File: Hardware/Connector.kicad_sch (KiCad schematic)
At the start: 13 parts, among them J1 XIAO ESP32S3 Sense, J2 Conn_02x16_Counter_Clockwise, J3 FTSH-107-01-L-D-K

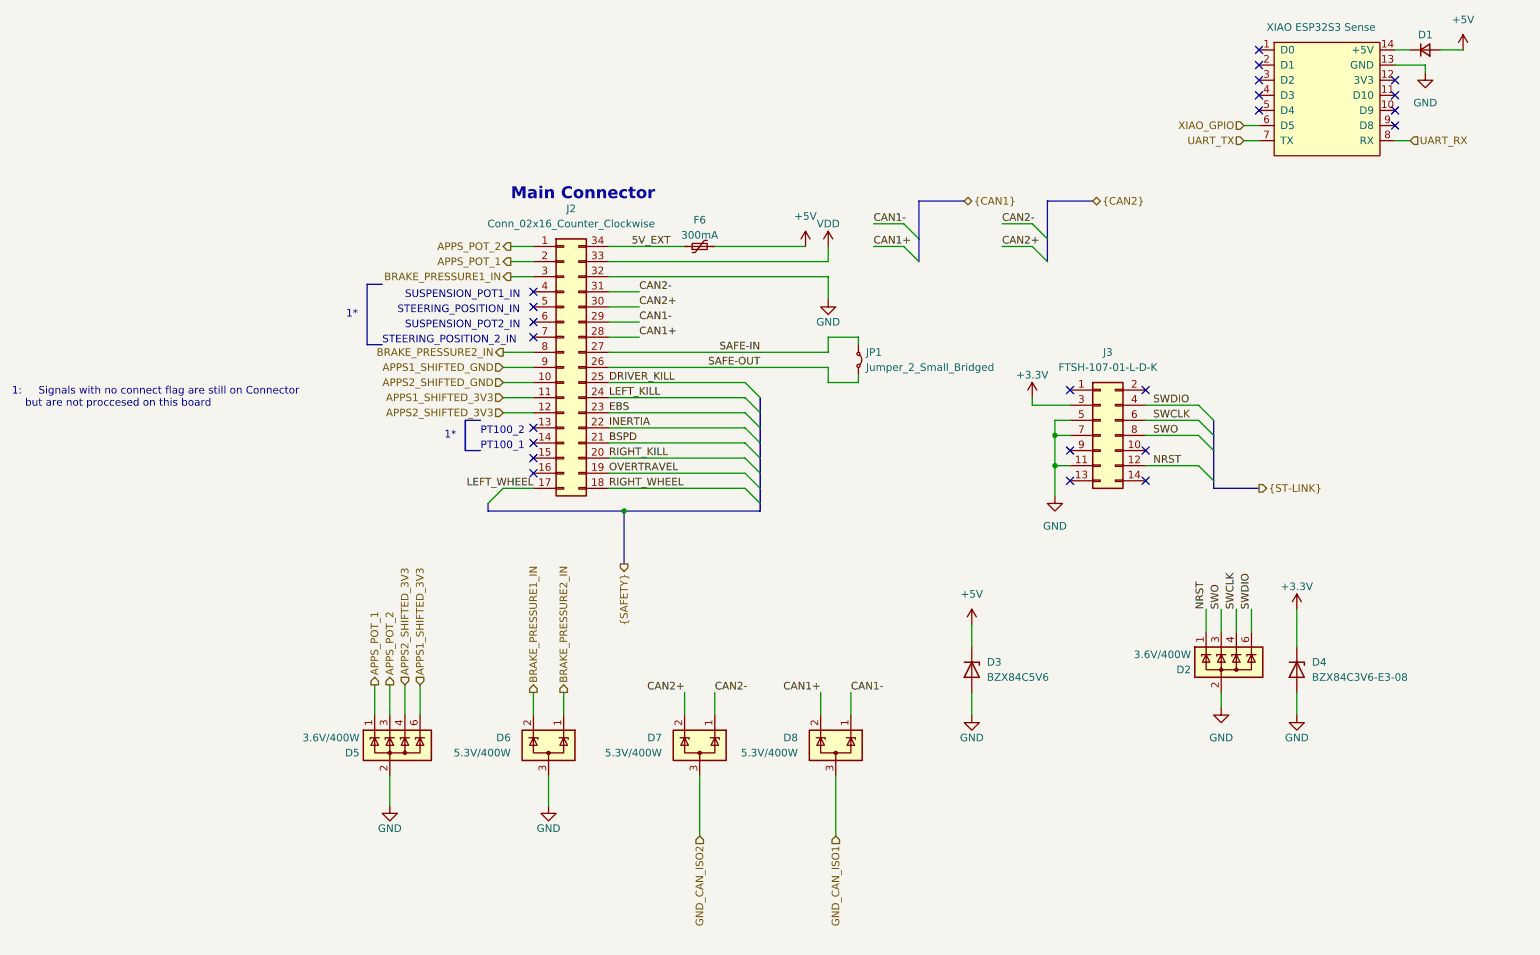
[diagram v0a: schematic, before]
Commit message: Initial routing (Piotruś proszę nie bij że brzydko)
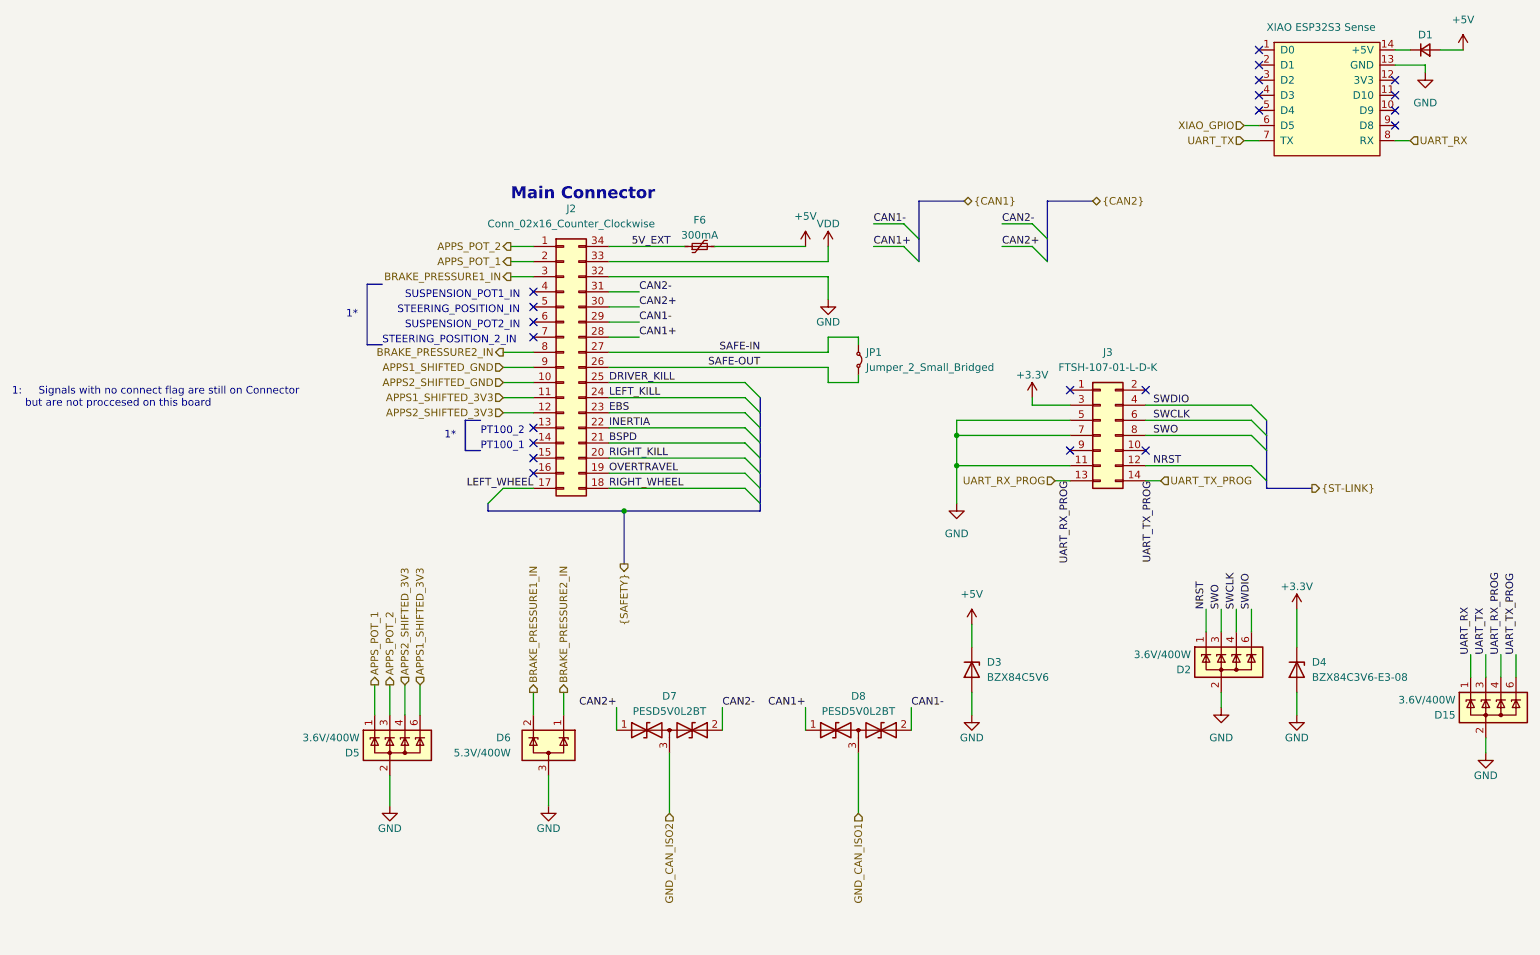
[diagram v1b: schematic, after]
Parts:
- removed D7, D8: 5.3V/400W, Package_TO_SOT_SMD:SOT-23-3, symbol Power_Protection:ESDA5V3L
- added D15: 3.6V/400W, Package_TO_SOT_SMD:SOT-23-6, symbol Power_Protection:ESDA5V3SC5
- added D7, D8: PESD5V0L2BT, Package_TO_SOT_SMD:SOT-23_Handsoldering, symbol Device:D_TVS_Dual_AAC
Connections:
- net CAN1+: now also D8.1 (A1)
- net CAN1-: now also D8.2 (A2)
- net CAN2+: now also D7.1 (A1)
- net CAN2-: now also D7.2 (A2)
- net GND: now also D15.2 (K), D15.5 (NC)
- net GND_CAN_ISO1: now also D8.3 (common)
- net GND_CAN_ISO2: now also D7.3 (common)
- net UART_RX: now also D15.1 (A)
- net UART_TX: now also D15.3 (A)
- net UART_RX_PROG: now reaches J3.13 (Pin_13)
- net UART_RX_PROG: now also D15.4 (A)
- net UART_TX_PROG: now reaches J3.14 (Pin_14)
- net UART_TX_PROG: now also D15.6 (A)
- no-connect marks 23 -> 21
